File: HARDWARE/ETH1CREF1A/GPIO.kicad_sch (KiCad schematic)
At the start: 10 parts, among them J1101 Conn_02x04_Odd_Even, U501 74HCT595PW, U503 SN74LVC1T45DRLR, U504 SN74LVC1T45DRLR, U505 SN74LVC1T45DRLR, U506 SN74LVC1T45DRLR

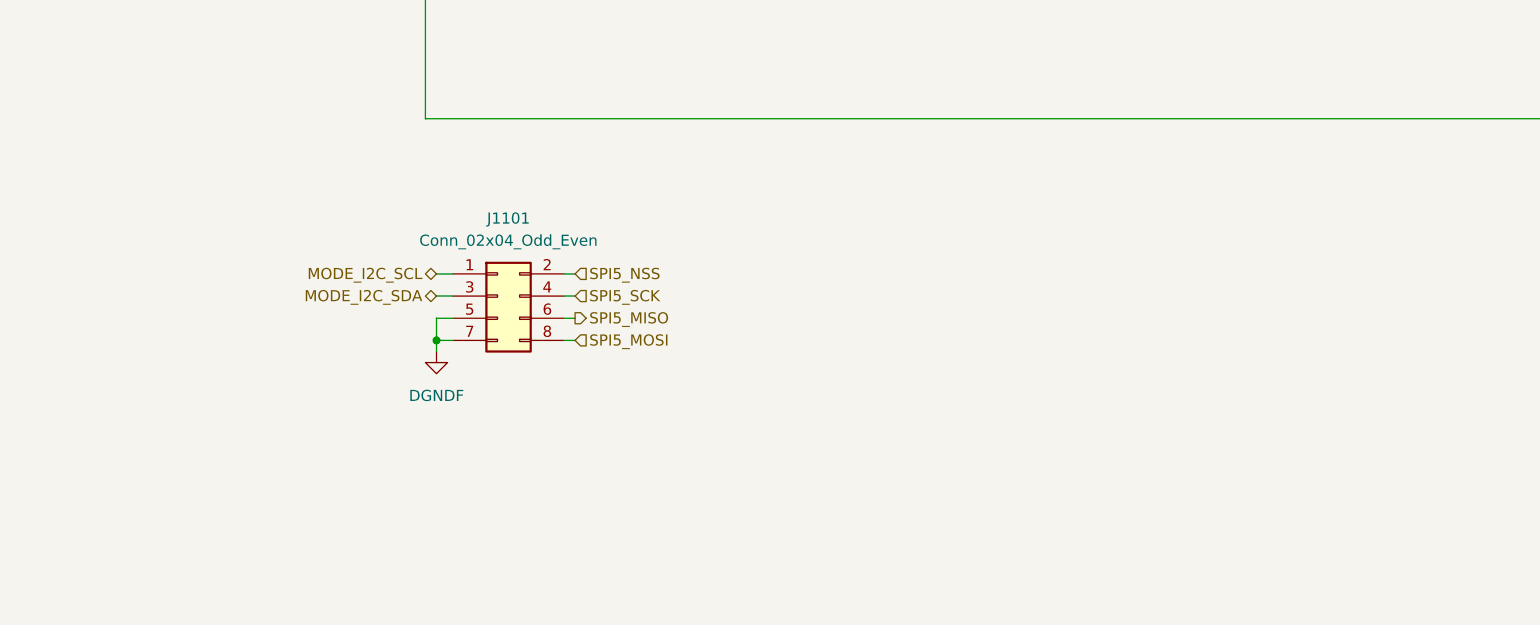
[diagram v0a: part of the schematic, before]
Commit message: Hardware
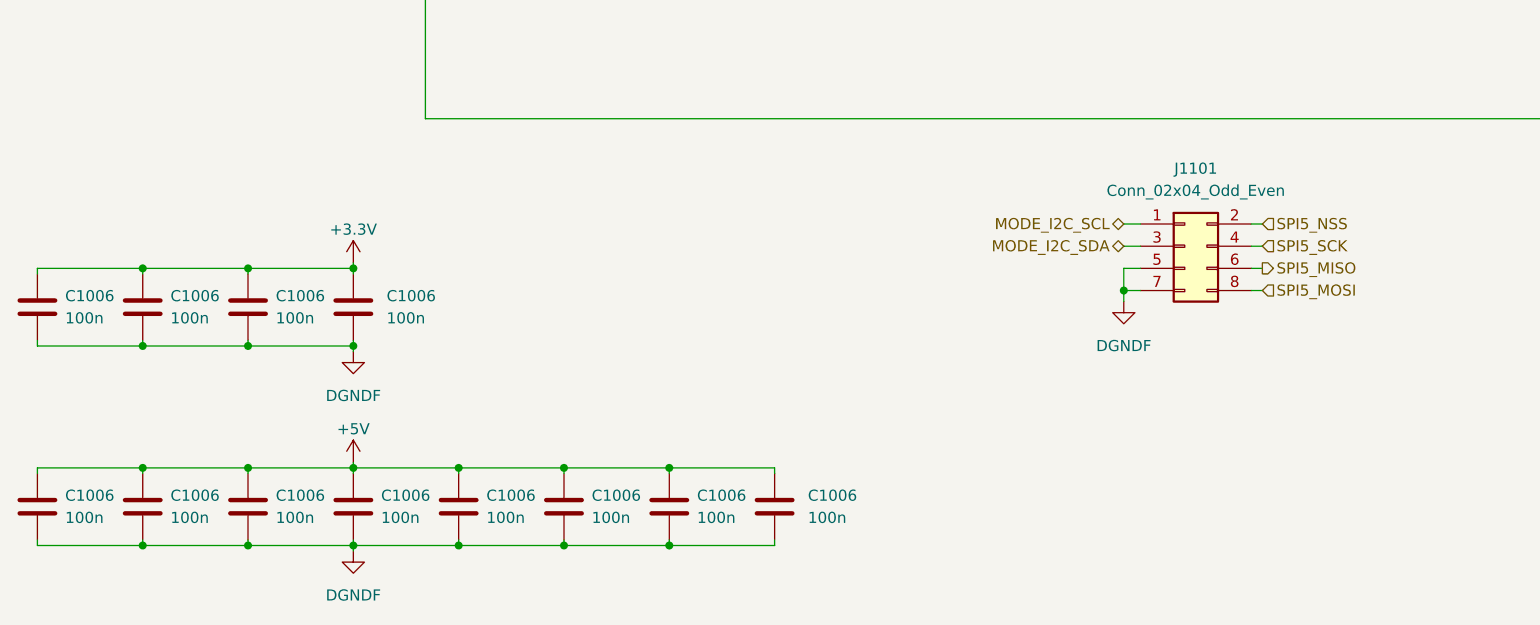
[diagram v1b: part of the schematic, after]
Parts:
- added C1006 (x12): 100n, Capacitor_SMD:C_0603_1608Metric_Pad1.08x0.95mm_HandSolder, symbol Device:C
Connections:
- net +3.3V: now also C1006.1, C1006.1, C1006.1, C1006.1
- net +5V: now also C1006.1, C1006.1, C1006.1, C1006.1, C1006.1, C1006.1, C1006.1, C1006.1
- net DGNDF: now also C1006.2, C1006.2, C1006.2, C1006.2, C1006.2, C1006.2, C1006.2, C1006.2, C1006.2, C1006.2, C1006.2, C1006.2
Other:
- moved on the sheet: J1101

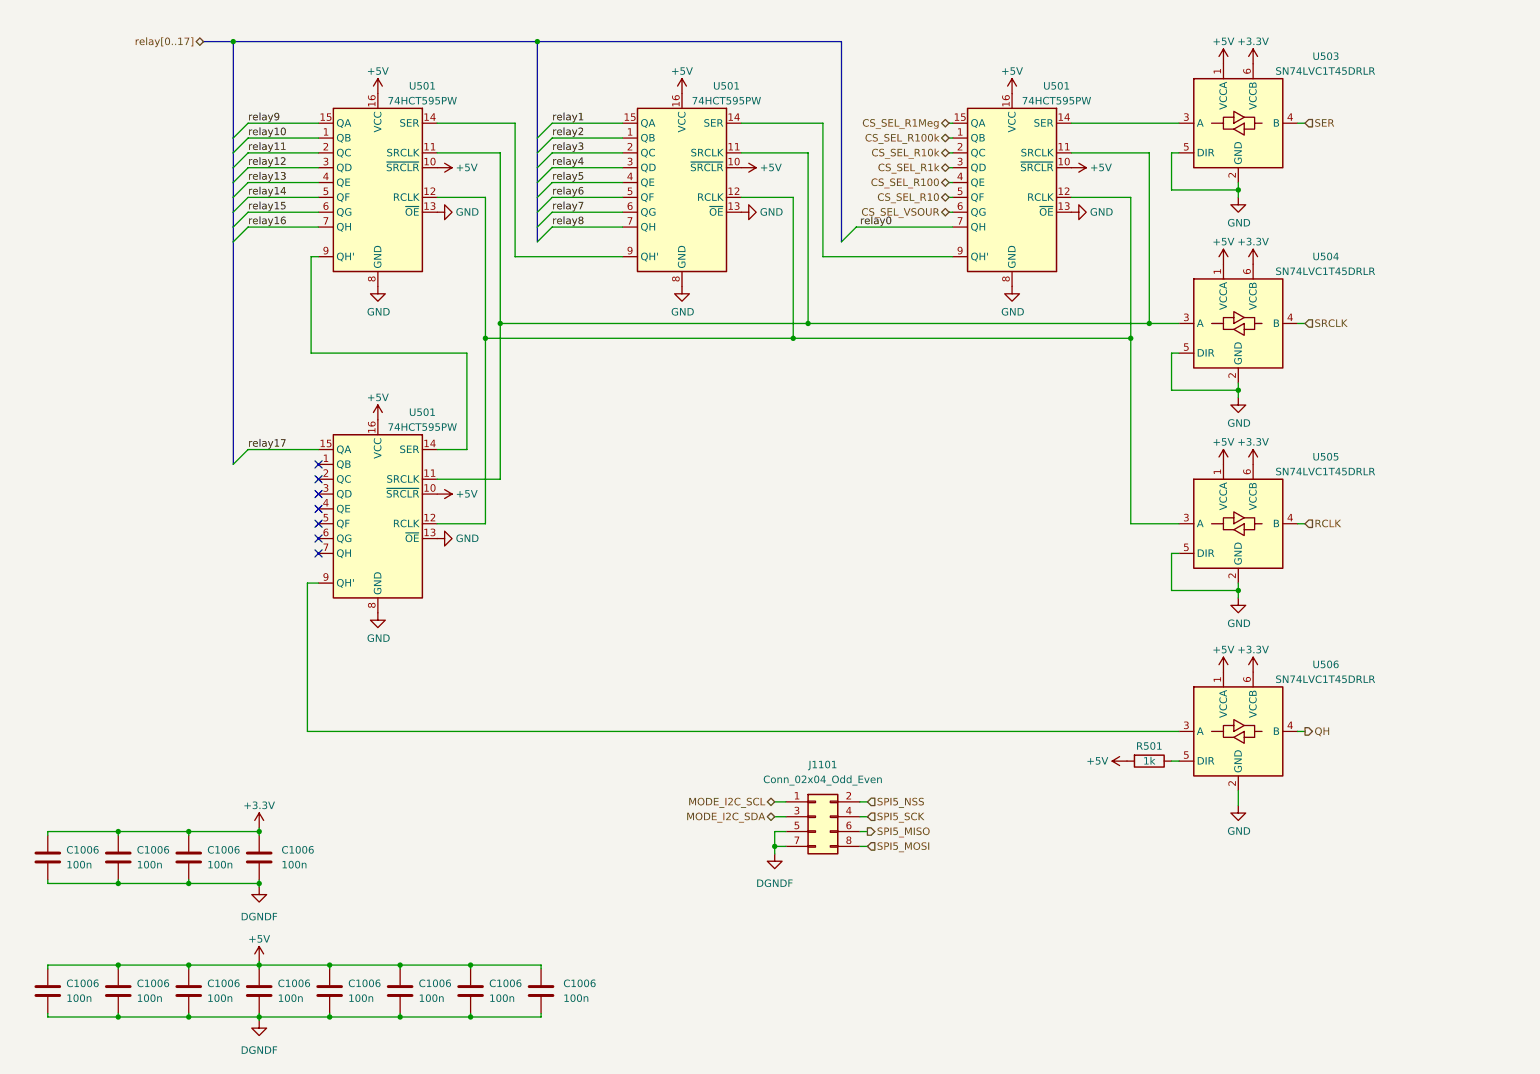
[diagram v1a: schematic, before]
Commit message: Hardware
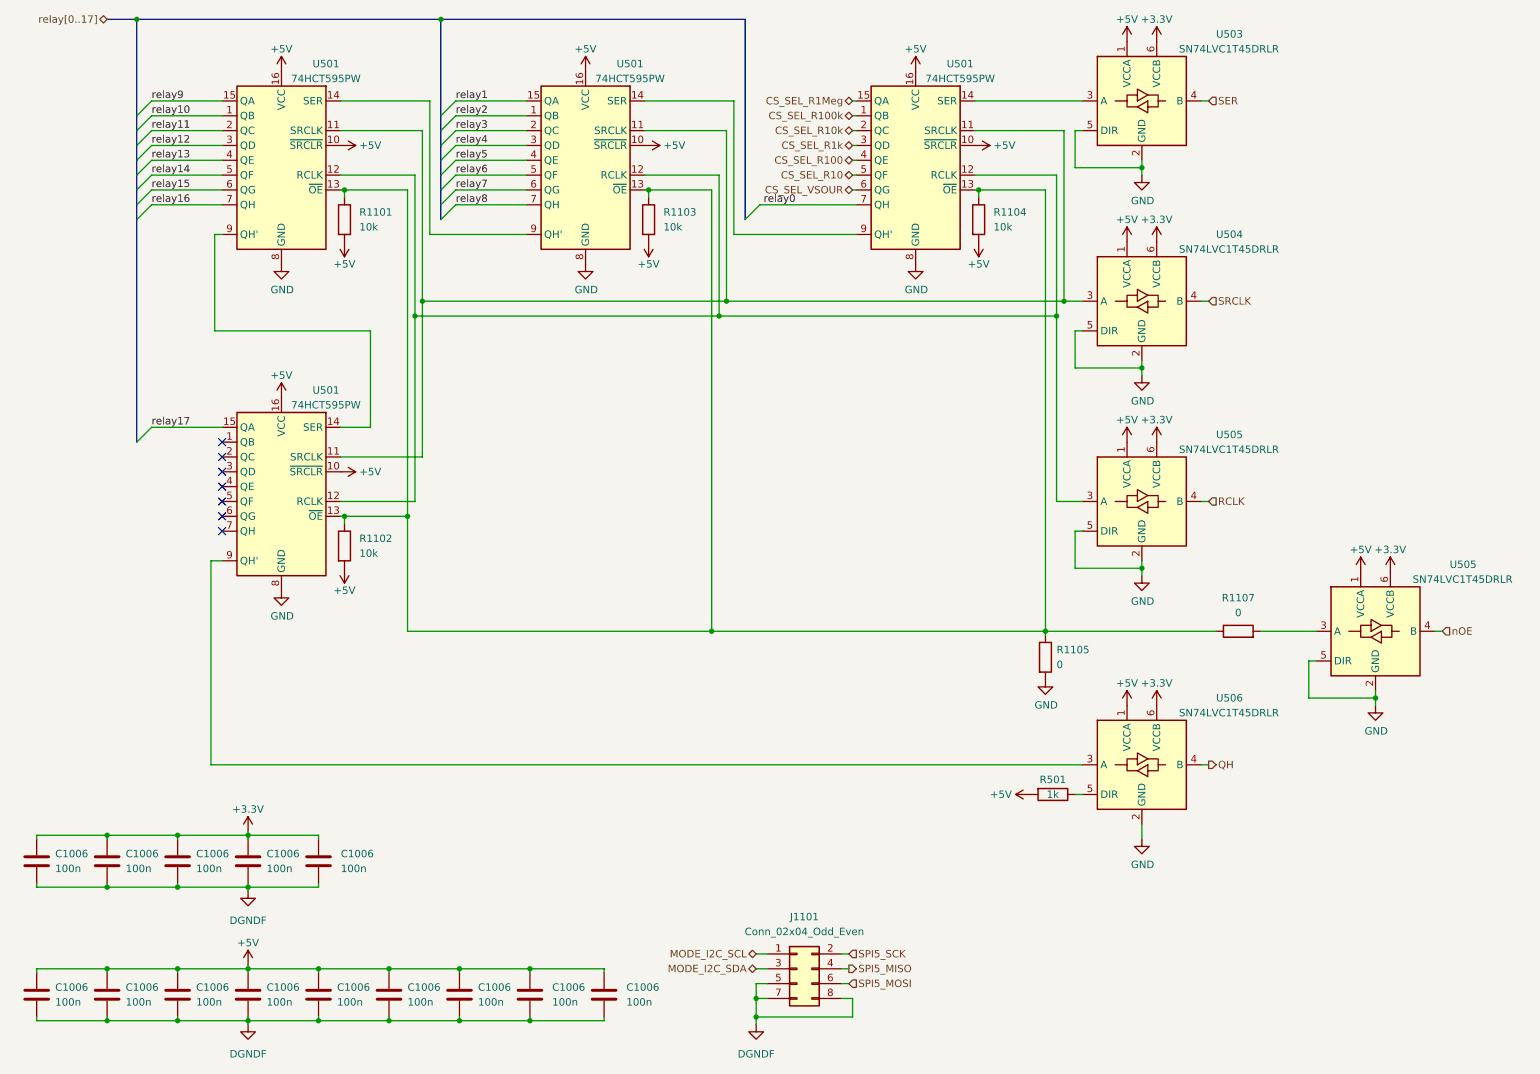
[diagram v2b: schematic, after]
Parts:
- added C1006 (x2): 100n, Capacitor_SMD:C_0603_1608Metric_Pad1.08x0.95mm_HandSolder, symbol Device:C
- added R1101, R1102, R1103, R1104: 10k, Resistor_SMD:R_0603_1608Metric_Pad0.98x0.95mm_HandSolder, symbol Device:R
- added R1105, R1107: 0, Resistor_SMD:R_0603_1608Metric_Pad0.98x0.95mm_HandSolder, symbol Device:R
- added U505: SN74LVC1T45DRLR, Package_TO_SOT_SMD:SOT-23-6, symbol Logic_LevelTranslator:SN74LVC1T45DBV
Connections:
- net SPI5_NSS is gone; now on net SPI5_SCK: J1101.2 (Pin_2)
- net +3.3V: now also C1006.1, U505.6 (VCCB)
- net +5V: now also C1006.1, R1101.2, R1102.2, R1103.2, R1104.2, U505.1 (VCCA)
- net DGNDF: now also J1101.8 (Pin_8), C1006.2, C1006.2
- net GND: now also R1105.2, U505.2 (GND), U505.5 (DIR); no longer U501.13 (~{OE}), U501.13 (~{OE}), U501.13 (~{OE}), U501.13 (~{OE})
- net SPI5_MISO: now also J1101.4 (Pin_4); no longer J1101.6 (Pin_6)
- net SPI5_MOSI: now also J1101.6 (Pin_6); no longer J1101.8 (Pin_8)
- net SPI5_SCK: no longer J1101.4 (Pin_4)
- new net: R1101.1, R1102.1, R1103.1, R1104.1, R1105.1, R1107.1, U501.13 (~{OE}), U501.13 (~{OE}), U501.13 (~{OE}), U501.13 (~{OE})
- new net: R1107.2, U505.3 (A)
- new net nOE: U505.4 (B)
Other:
- moved on the sheet: C1006, J1101, R501, U501, U503, U504, U505, U506

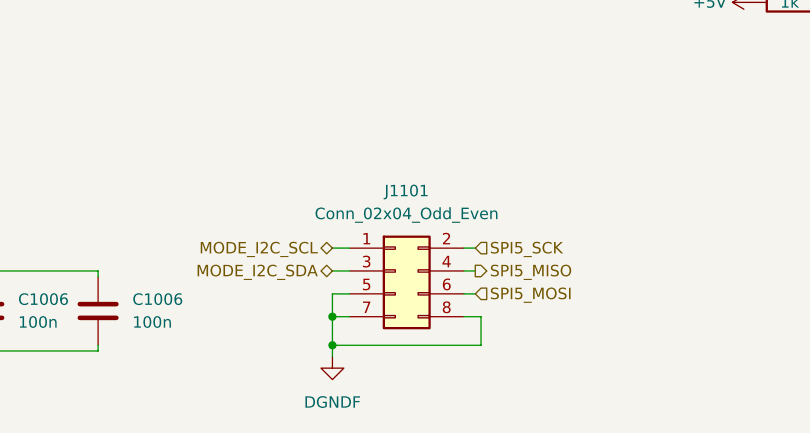
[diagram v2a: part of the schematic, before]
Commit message: Hardware
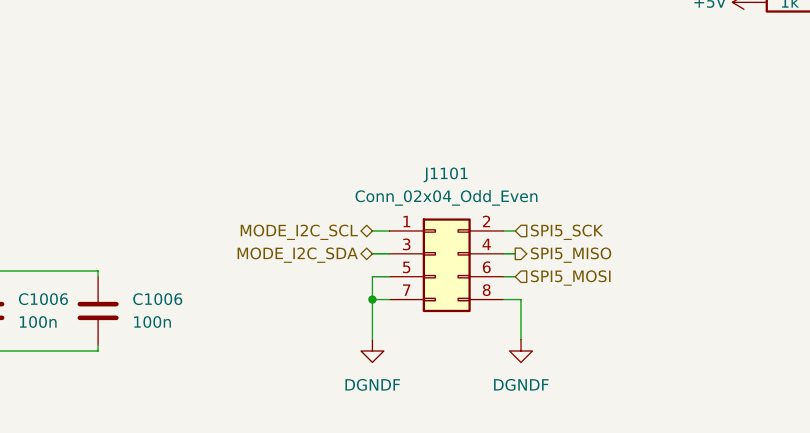
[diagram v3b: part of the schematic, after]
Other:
- moved on the sheet: J1101
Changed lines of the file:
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@@
   (junction (at 136.525 66.675) (diameter 0) (color 0 0 0 0)
   )
-  (junction (at 141.605 186.055) (diameter 0) (color 0 0 0 0)
+  (junction (at 146.05 184.15) (diameter 0) (color 0 0 0 0)
   )
   (junction (at 42.545 167.005) (diameter 0) (color 0 0 0 0)
-  )
-  (junction (at 141.605 189.23) (diameter 0) (color 0 0 0 0)
   )
   (junction (at 78.74 189.865) (diameter 0) (color 0 0 0 0)
@@
     (stroke (width 0) (type default))
   )
-  (wire (pts (xy 141.605 189.23) (xy 158.115 189.23))
-    (stroke (width 0) (type default))
-  )
   (wire (pts (xy 196.215 112.395) (xy 196.215 106.045))
     (stroke (width 0) (type default))
@@
     (stroke (width 0) (type default))
   )
-  (wire (pts (xy 141.605 189.23) (xy 141.605 186.055))
+  (wire (pts (xy 146.05 184.15) (xy 146.05 188.595))
     (stroke (width 0) (type default))
   )
@@
     (stroke (width 0) (type default))
   )
-  (wire (pts (xy 158.115 186.055) (xy 156.21 186.055))
+  (wire (pts (xy 162.56 184.15) (xy 160.655 184.15))
     (stroke (width 0) (type default))
   )
@@
     (stroke (width 0) (type default))
   )
-  (wire (pts (xy 141.605 183.515) (xy 143.51 183.515))
+  (wire (pts (xy 146.05 181.61) (xy 147.955 181.61))
     (stroke (width 0) (type default))
   )
@@
     (stroke (width 0) (type default))
   )
-  (wire (pts (xy 158.115 189.23) (xy 158.115 186.055))
+  (wire (pts (xy 162.56 188.595) (xy 162.56 184.15))
     (stroke (width 0) (type default))
   )
@@
     (stroke (width 0) (type default))
   )
-  (wire (pts (xy 141.605 178.435) (xy 143.51 178.435))
+  (wire (pts (xy 146.05 176.53) (xy 147.955 176.53))
     (stroke (width 0) (type default))
   )
@@
     (stroke (width 0) (type default))
   )
-  (wire (pts (xy 157.48 183.515) (xy 156.21 183.515))
+  (wire (pts (xy 161.925 181.61) (xy 160.655 181.61))
     (stroke (width 0) (type default))
   )
@@
     (stroke (width 0) (type default))
   )
-  (wire (pts (xy 157.48 180.975) (xy 156.21 180.975))
-    (stroke (width 0) (type default))
-  )
-  (wire (pts (xy 141.605 186.055) (xy 141.605 183.515))
+  (wire (pts (xy 161.925 179.07) (xy 160.655 179.07))
+    (stroke (width 0) (type default))
+  )
+  (wire (pts (xy 146.05 184.15) (xy 146.05 181.61))
     (stroke (width 0) (type default))
   )
@@
     (stroke (width 0) (type default))
   )
-  (wire (pts (xy 141.605 180.975) (xy 143.51 180.975))
+  (wire (pts (xy 146.05 179.07) (xy 147.955 179.07))
     (stroke (width 0) (type default))
   )
@@
     (stroke (width 0) (type default))
   )
-  (wire (pts (xy 157.48 178.435) (xy 156.21 178.435))
+  (wire (pts (xy 161.925 176.53) (xy 160.655 176.53))
     (stroke (width 0) (type default))
   )
@@
     (stroke (width 0) (type default))
   )
-  (wire (pts (xy 141.605 186.055) (xy 143.51 186.055))
+  (wire (pts (xy 146.05 184.15) (xy 147.955 184.15))
     (stroke (width 0) (type default))
   )
@@
   )
   (bus (pts (xy 139.7 18.415) (xy 87.63 18.415))
-    (stroke (width 0) (type default))
-  )
-  (wire (pts (xy 141.605 190.5) (xy 141.605 189.23))
     (stroke (width 0) (type default))
   )
@@
     (effects (font (size 1.27 1.27)) (justify left))
   )
-  (hierarchical_label "SPI5_MISO" (shape output) (at 157.48 180.975 0) (fields_autoplaced)
+  (hierarchical_label "SPI5_MISO" (shape output) (at 161.925 179.07 0) (fields_autoplaced)
     (effects (font (size 1.27 1.27)) (justify left))
   )
@@
     (effects (font (size 1.27 1.27)) (justify right))
   )
-  (hierarchical_label "MODE_I2C_SCL" (shape bidirectional) (at 141.605 178.435 180) (fields_autoplaced)
+  (hierarchical_label "MODE_I2C_SCL" (shape bidirectional) (at 146.05 176.53 180) (fields_autoplaced)
     (effects (font (size 1.27 1.27)) (justify right))
   )
@@
     (effects (font (size 1.27 1.27)) (justify left))
   )
-  (hierarchical_label "MODE_I2C_SDA" (shape bidirectional) (at 141.605 180.975 180) (fields_autoplaced)
+  (hierarchical_label "MODE_I2C_SDA" (shape bidirectional) (at 146.05 179.07 180) (fields_autoplaced)
     (effects (font (size 1.27 1.27)) (justify right))
   )
@@
     (effects (font (size 1.27 1.27)) (justify right))
   )
-  (hierarchical_label "SPI5_SCK" (shape input) (at 157.48 178.435 0) (fields_autoplaced)
+  (hierarchical_label "SPI5_SCK" (shape input) (at 161.925 176.53 0) (fields_autoplaced)
     (effects (font (size 1.27 1.27)) (justify left))
   )
-  (hierarchical_label "SPI5_MOSI" (shape input) (at 157.48 183.515 0) (fields_autoplaced)
+  (hierarchical_label "SPI5_MOSI" (shape input) (at 161.925 181.61 0) (fields_autoplaced)
     (effects (font (size 1.27 1.27)) (justify left))
   )
@@
     )
   )
-  (symbol (lib_id "ETH1CREF1A:DGNDF") (at 141.605 190.5 0) (unit 1)
+  (symbol (lib_id "ETH1CREF1A:DGNDF") (at 146.05 188.595 0) (unit 1)
     (in_bom yes) (on_board yes) (dnp no) (fields_autoplaced)
-    (property "Reference" "#PWR01117" (at 141.605 196.85 0)
-      (effects (font (size 1.27 1.27)) hide)
-    )
-    (property "Value" "DGNDF" (at 141.605 195.58 0)
-      (effects (font (size 1.27 1.27)))
-    )
-    (property "Footprint" "" (at 141.605 190.5 0)
-      (effects (font (size 1.27 1.27)) hide)
-    )
-    (property "Datasheet" "" (at 141.605 190.5 0)
+    (property "Reference" "#PWR01117" (at 146.05 194.945 0)
+      (effects (font (size 1.27 1.27)) hide)
+    )
+    (property "Value" "DGNDF" (at 146.05 193.675 0)
+      (effects (font (size 1.27 1.27)))
+    )
+    (property "Footprint" "" (at 146.05 188.595 0)
+      (effects (font (size 1.27 1.27)) hide)
+    )
+    (property "Datasheet" "" (at 146.05 188.595 0)
       (effects (font (size 1.27 1.27)) hide)
     )
@@
     )
   )
-  (symbol (lib_id "Connector_Generic:Conn_02x04_Odd_Even") (at 148.59 180.975 0) (unit 1)
+  (symbol (lib_id "Connector_Generic:Conn_02x04_Odd_Even") (at 153.035 179.07 0) (unit 1)
     (in_bom yes) (on_board yes) (dnp no) (fields_autoplaced)
-    (property "Reference" "J1101" (at 149.86 172.085 0)
-      (effects (font (size 1.27 1.27)))
-    )
-    (property "Value" "Conn_02x04_Odd_Even" (at 149.86 174.625 0)
-      (effects (font (size 1.27 1.27)))
-    )
-    (property "Footprint" "Connector_PinHeader_2.54mm:PinHeader_2x04_P2.54mm_Vertical" (at 148.59 180.975 0)
-      (effects (font (size 1.27 1.27)) hide)
-    )
-    (property "Datasheet" "~" (at 148.59 180.975 0)
+    (property "Reference" "J1101" (at 154.305 170.18 0)
+      (effects (font (size 1.27 1.27)))
+    )
+    (property "Value" "Conn_02x04_Odd_Even" (at 154.305 172.72 0)
+      (effects (font (size 1.27 1.27)))
+    )
+    (property "Footprint" "Connector_PinHeader_2.54mm:PinHeader_2x04_P2.54mm_Vertical" (at 153.035 179.07 0)
+      (effects (font (size 1.27 1.27)) hide)
+    )
+    (property "Datasheet" "~" (at 153.035 179.07 0)
       (effects (font (size 1.27 1.27)) hide)
     )
@@
         )
       )
+    )
+  )
+  (symbol (lib_id "ETH1CREF1A:DGNDF") (at 162.56 188.595 0) (unit 1)
+    (in_bom yes) (on_board yes) (dnp no) (fields_autoplaced)
+    (property "Reference" "#PWR01139" (at 162.56 194.945 0)
+      (effects (font (size 1.27 1.27)) hide)
+    )
+    (property "Value" "DGNDF" (at 162.56 193.675 0)
+      (effects (font (size 1.27 1.27)))
+    )
+    (property "Footprint" "" (at 162.56 188.595 0)
+      (effects (font (size 1.27 1.27)) hide)
+    )
+    (property "Datasheet" "" (at 162.56 188.595 0)
+      (effects (font (size 1.27 1.27)) hide)
+    )
+    (pin "1")
+    (instances
+      (project "ETH1CREF1A"
+        (path "/f534bde3-7724-4aa2-8c73-8f0531e01e95/480dccee-21e0-4e1b-a4b7-7a66648dd9b9"
+          (reference "#PWR01139") (unit 1)
+        )
+      )
